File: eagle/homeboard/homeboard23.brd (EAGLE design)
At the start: 94 x 71.8 mm, 128 parts, among them IC1 XCF02S, IC2 25LC080SN, IC3 ATMEGA32U2-TQFP, Q5 BC848SMD, Q6 BC848SMD, Q7 BC848SMD, Q8 BC848SMD, T1 BSS138, T2 BC848, T3 BSS138, U1 XC3S400TQ144, X1 SCART-CLIP, X6 MINI-USB_4P-85-32004-10X, X7 DC21MMX, X8 STEREOJACK

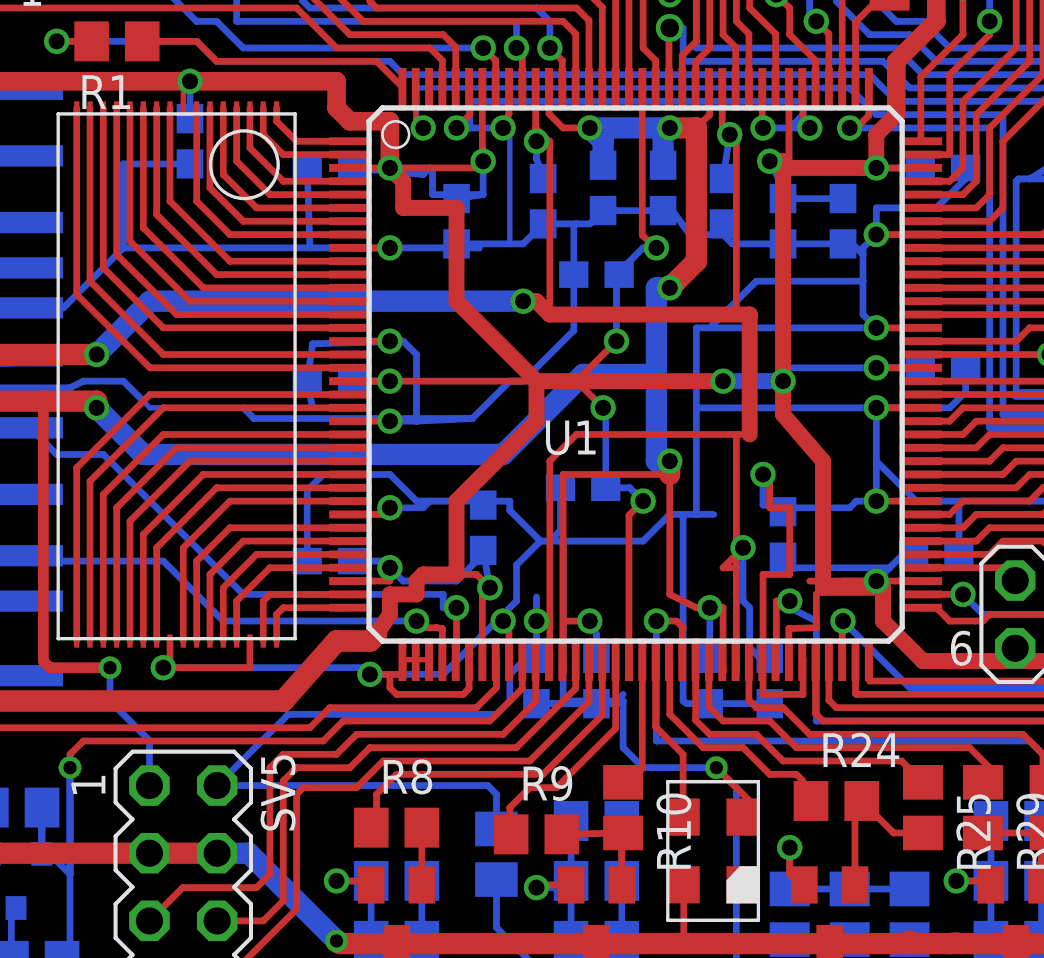
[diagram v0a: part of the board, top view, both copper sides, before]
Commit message: more
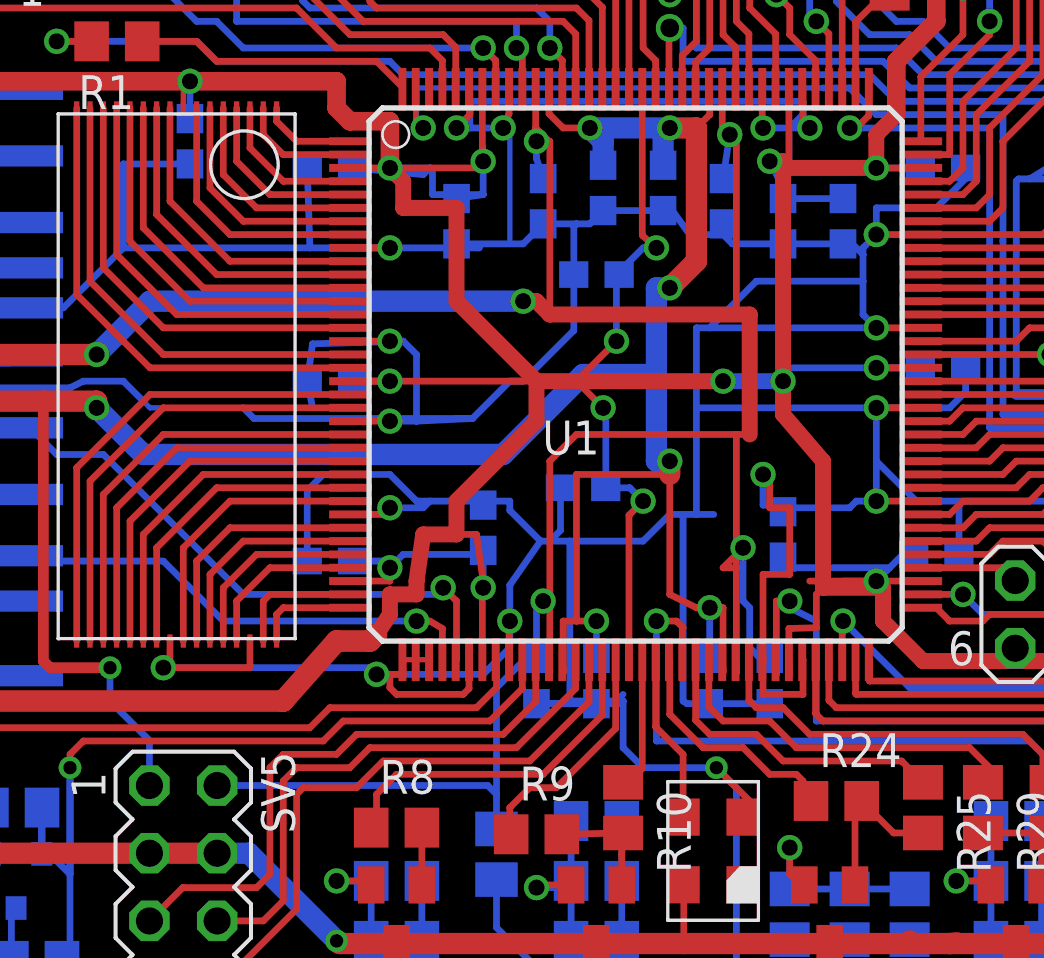
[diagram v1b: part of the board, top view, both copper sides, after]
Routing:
- net VCCAUX: track 141.7 -> 132.9 mm
- net VCC: track 557.5 -> 558.5 mm
